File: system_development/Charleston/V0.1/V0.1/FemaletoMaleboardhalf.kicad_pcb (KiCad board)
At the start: 2 copper layers, 36.1 x 64.4 mm, 4 parts, among them J1 Screw_Terminal_01x12

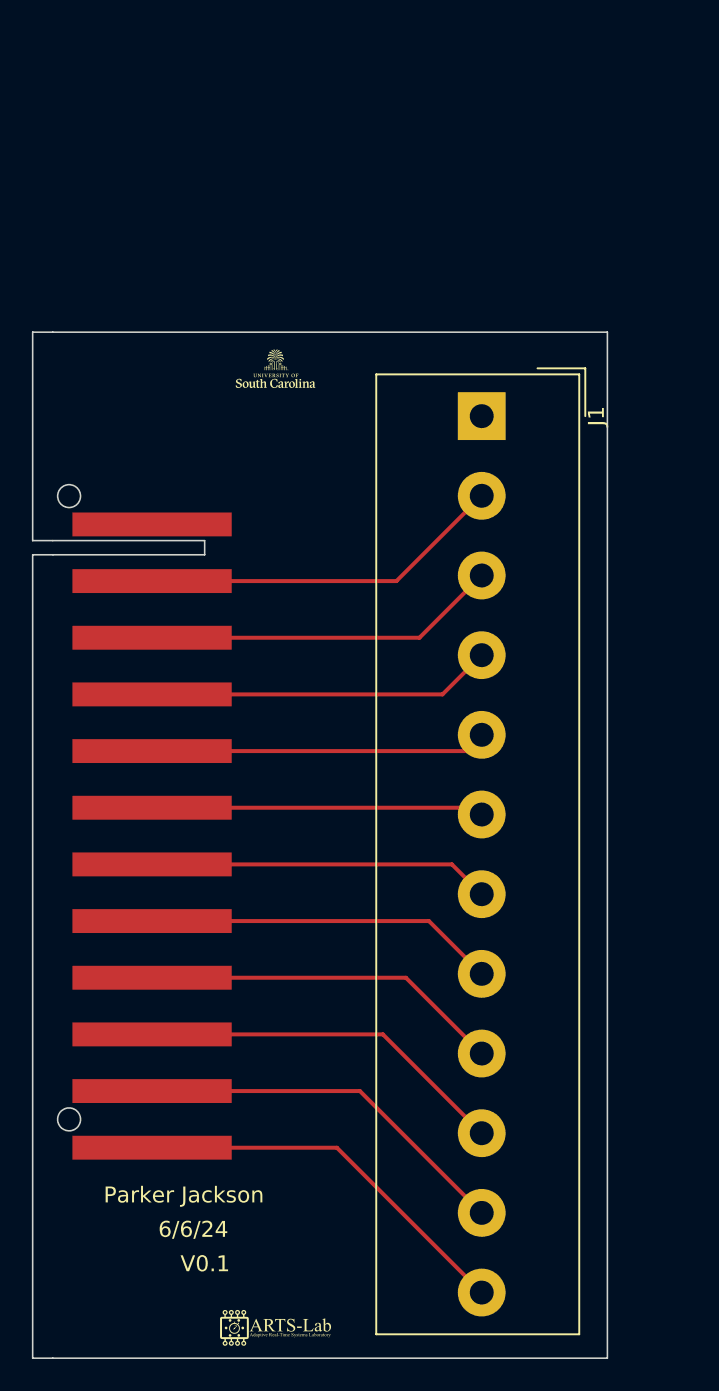
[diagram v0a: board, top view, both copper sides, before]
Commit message: Updated Read me
trying

trying

reverting to before I messed up librarys

reverting to before I messed up librarys

reverting to before I messed up librarys

reverting to before I messed up librarys

reverting to before I messed up librarys

reverting to before I messed up librarys

Fixed all issues

Fixed all issues

Fixed all issues

Fixed all issues

Updated Readme

Updated Readme

Updated Readme

Updated Readme
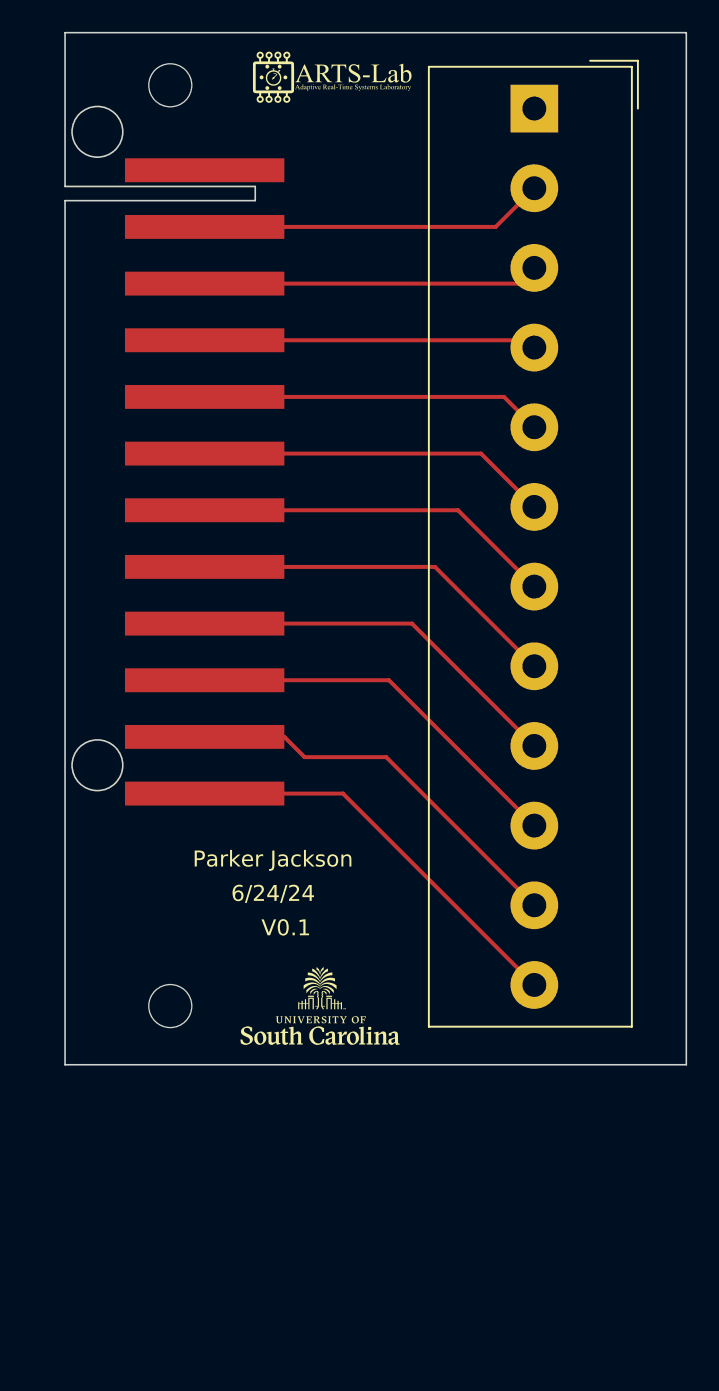
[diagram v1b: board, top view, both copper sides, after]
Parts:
- added REF**: MountingHole_2.7mm, MountingHole:MountingHole_2.7mm, F.Cu at (117.2, 45.6)
- added REF**: MountingHole_2.7mm, MountingHole:MountingHole_2.7mm, F.Cu at (117.2, 103.4)
- moved G*** 78.6 mm to (127.4, 45.1)
- moved G*** 40.1 mm to (126.6, 103.4)
- moved U1 22.5 mm to (125.0, 70.5)
- moved J1 19.6 mm to (140.1, 47.1)
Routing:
- net Net-(J1-Pin_10): track 0.00 -> 24.5 mm
- net Net-(J1-Pin_11): track 47.1 -> 25.1 mm
- net Net-(J1-Pin_5): track 0.00 -> 21.5 mm
- net Net-(J1-Pin_6): track 42.0 -> 22.1 mm
- net Net-(J1-Pin_9): track 22.7 -> 23.9 mm
- net Net-(J1-Pin_8): track 22.1 -> 23.3 mm
- net Net-(J1-Pin_7): track 21.5 -> 22.7 mm
- net Net-(J1-Pin_3): track 22.3 -> 21.1 mm
- net Net-(J1-Pin_2): track 22.9 -> 21.7 mm
- net Net-(J1-Pin_12): track 24.5 -> 25.7 mm
- net Net-(J1-Pin_4): track 21.7 -> 20.9 mm
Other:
- board size 36.1 x 64.4 mm -> 39 x 64.8 mm
- board text added: "6/24/24"
- board text removed: "6/6/24"
